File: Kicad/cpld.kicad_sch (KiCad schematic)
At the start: 16 parts, among them J2 Conn_01x06_Pin, U7 AMS1117-3.3, U9 XC95144XL-TQ144

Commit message: Fix LCSC parts issues
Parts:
- FB6, FB7, FB8: LCSC Part # (none) -> C95177
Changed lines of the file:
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@@
 			)
 		)
-		(property "LCSC Part #" ""
+		(property "LCSC Part #" "C95177"
 			(at 111.76 68.58 90)
 			(effects
@@
 			)
 		)
-		(property "LCSC Part #" ""
+		(property "LCSC Part #" "C95177"
 			(at 111.76 154.94 90)
 			(effects
@@
 			)
 		)
-		(property "LCSC Part #" ""
+		(property "LCSC Part #" "C95177"
 			(at 111.76 144.78 90)
 			(effects

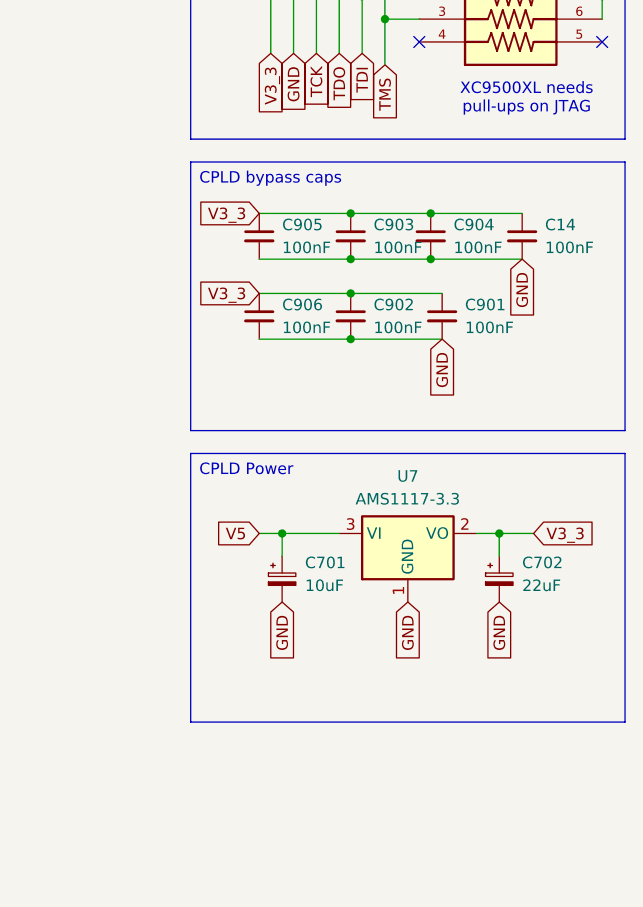
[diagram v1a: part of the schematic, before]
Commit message: Clean up schematics
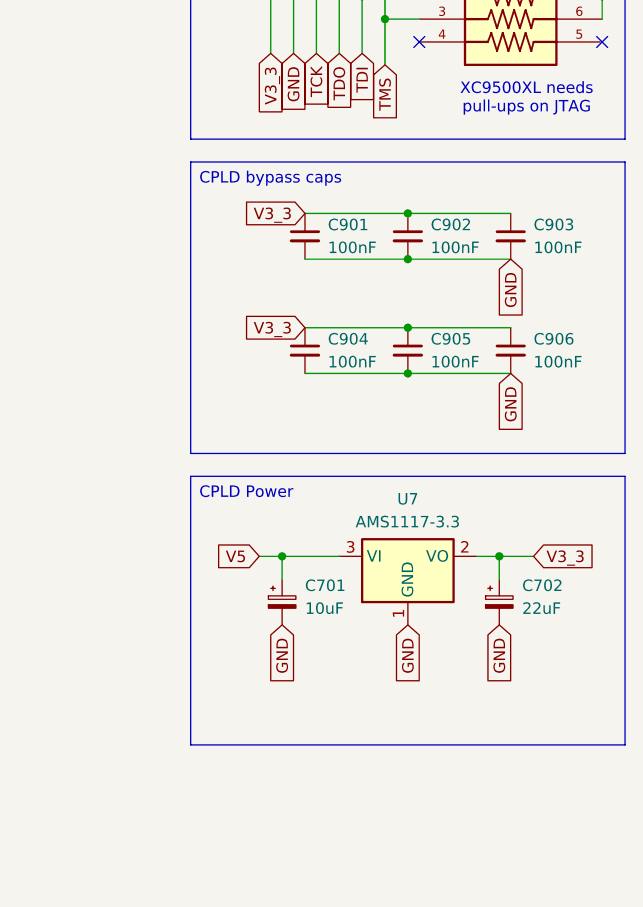
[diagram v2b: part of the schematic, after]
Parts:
- removed C14: 100nF, Capacitor_SMD:C_0603_1608Metric_Pad1.08x0.95mm_HandSolder, symbol Device:C_Small
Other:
- moved on the sheet: C701, C702, C901, C902, C903, C904, C905, C906, U7
